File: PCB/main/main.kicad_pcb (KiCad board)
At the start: 2 copper layers, 82.3 x 36.1 mm, 38 parts, among them IC1 LT8316IFE#PBF, Q1 PBHV9050ZF, Q2 IXTA10P50P, Q3 SIHB24N80AE-GE3, T1 Transformer_1P_2S

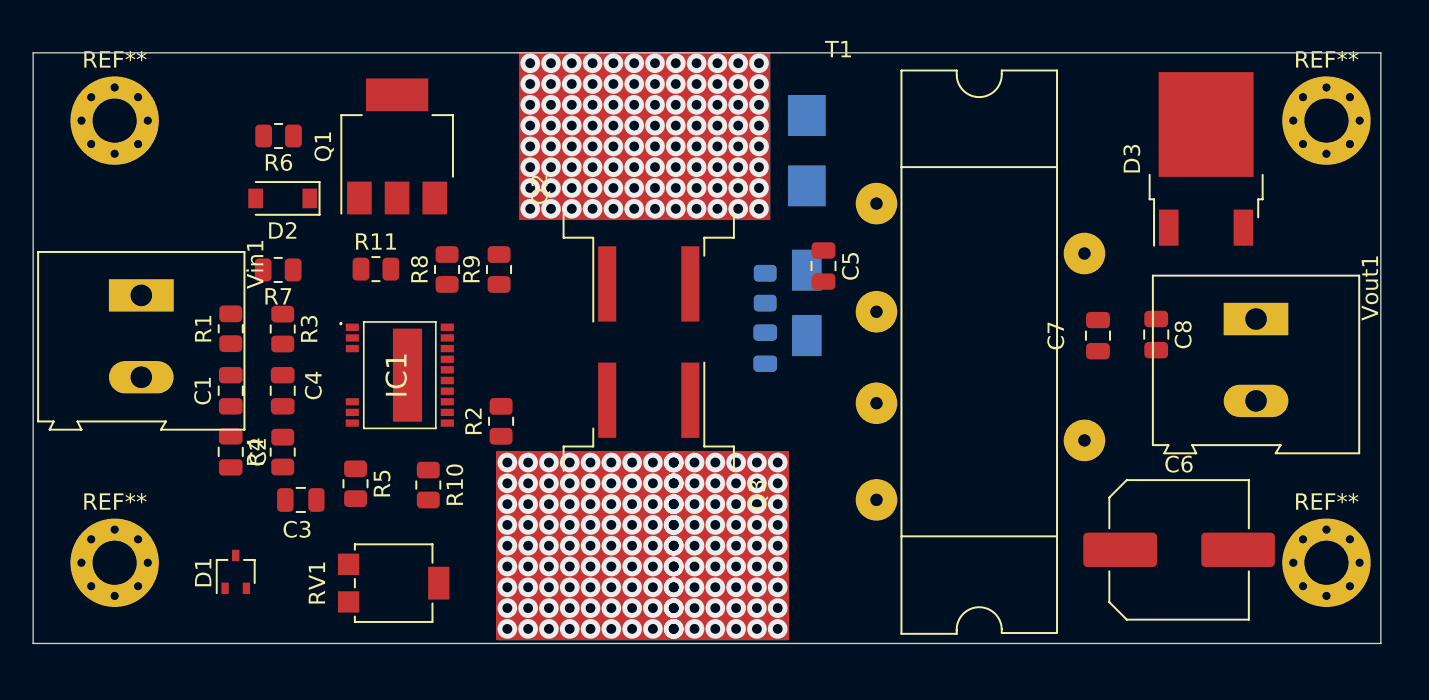
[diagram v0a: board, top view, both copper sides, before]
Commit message: pcb drawing update
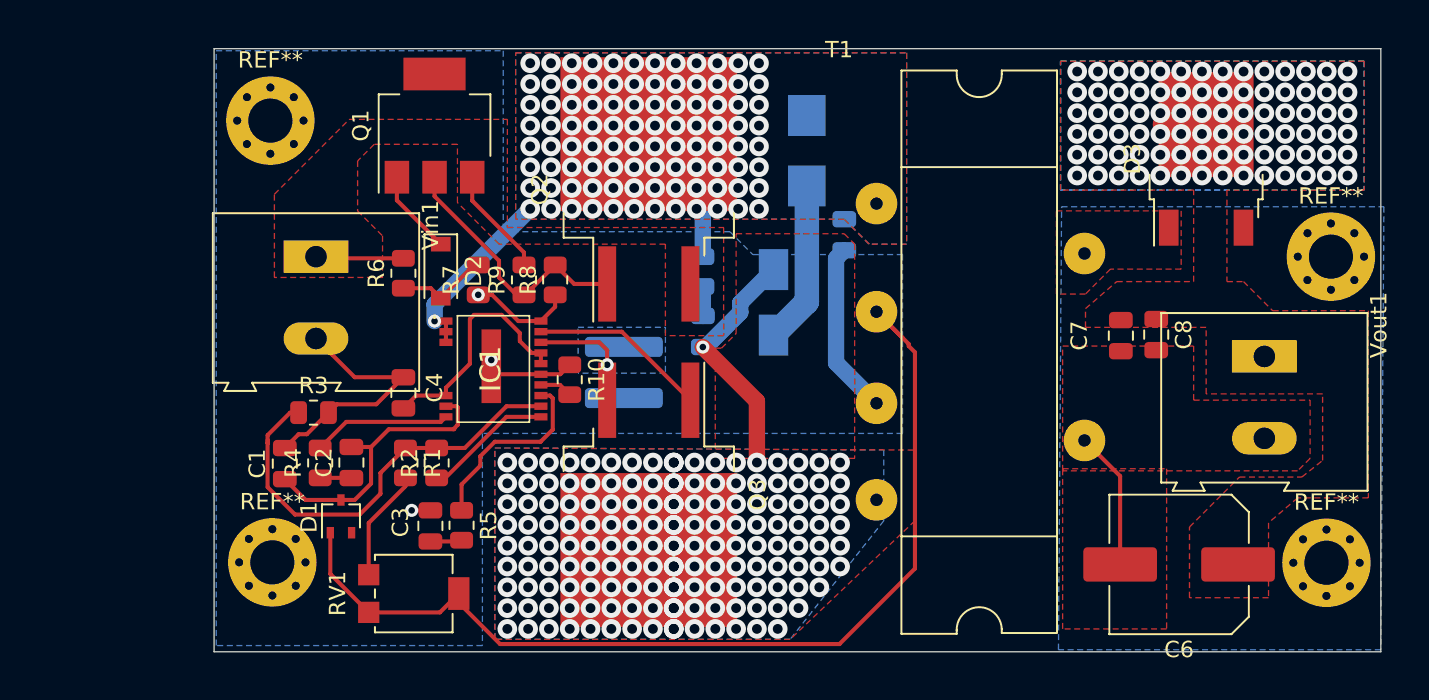
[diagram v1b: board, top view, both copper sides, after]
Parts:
- C5: moved to B.Cu
- R11: footprint Resistor_SMD:R_0805_2012Metric -> Resistor_SMD:R_1218_3246Metric_Pad1.22x4.75mm_HandSolder; moved to B.Cu
- moved R11 16.4 mm to (101.1, 42.4), turned to 90 degrees
- moved R1 13.5 mm to (87.8, 47.9), turned to 270 degrees
- moved R7 12.2 mm to (92.2, 36.7), turned to 90 degrees
- moved R6 11.3 mm to (87.6, 36.3), turned to 90 degrees
- moved Vin1 10.9 mm to (82.3, 35.3)
- moved R10 10.8 mm to (97.8, 42.8)
- moved D2 10.6 mm to (89.9, 36.2), turned to 270 degrees
- moved REF** 9.63 mm to (79.6, 54.0)
- moved REF** 9.51 mm to (79.5, 27.0)
- moved REF** 8.31 mm to (144.3, 35.3)
- moved C3 8.07 mm to (89.3, 51.8), turned to 270 degrees
- moved C2 7.39 mm to (84.5, 47.9), turned to 90 degrees
- moved C4 7.37 mm to (87.6, 43.6)
- moved D1 7.27 mm to (83.8, 51.2)
- moved R5 6.96 mm to (91.2, 51.7)
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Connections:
- D3 pad 1: Net-(C6-Pad1) -> Net-(D3-Pad1)
- D3 pad 2: Net-(D3-Pad2) -> Net-(C6-Pad1)
- D5 pad 1: Net-(D4-Pad1) -> Net-(C9-Pad2)
- D5 pad 2: Net-(C9-Pad2) -> Net-(D4-Pad1)
- T1 pad 3: Net-(D3-Pad2) -> Net-(D3-Pad1)
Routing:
- net V_FB: track 0.00 -> 62.1 mm
- net GND1: track 0.00 -> 42.0 mm, vias 0 -> 3
- net Net-(IC1-Pad12): track 0.00 -> 26.7 mm
- net Net-(C1-Pad1): track 0.00 -> 17.4 mm
- net Net-(Q1-Pad2): track 0.00 -> 16.0 mm
- net Net-(C9-Pad2): track 0.00 -> 15.0 mm, vias 80 -> 157
- net Net-(C4-Pad1): track 0.00 -> 14.5 mm
- net V_in: track 0.00 -> 14.4 mm, vias 71 -> 96
- net Net-(Q1-Pad3): track 0.00 -> 12.0 mm
- net Net-(IC1-Pad13): track 0.00 -> 11.6 mm
- net Net-(IC1-Pad19): track 0.00 -> 10.9 mm
- net Net-(D4-Pad1): track 0.00 -> 9.95 mm
- net Net-(IC1-Pad18): track 0.00 -> 9.85 mm, vias 0 -> 1
- net Net-(C6-Pad2): track 0.00 -> 8.47 mm
- net Net-(IC1-Pad10): track 0.00 -> 8.47 mm
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- added copper zone on B.Cu, net GND1
- added copper zone on B.Cu, net Net-(C6-Pad1)
- added copper zone on F.Cu, net Net-(C6-Pad1)
- added copper zone on B.Cu, net Net-(C6-Pad2)
- added copper zone on F.Cu, net Net-(C6-Pad2)
- added copper zone on B.Cu, net Net-(C9-Pad2)
- added copper zone on F.Cu, net Net-(C9-Pad2)
- added copper zone on F.Cu, net Net-(D3-Pad1)
- added copper zone on B.Cu, net Net-(D3-Pad2)
- added copper zone on B.Cu, net Net-(IC1-Pad18)
- added copper zone on F.Cu, net Net-(Q1-Pad3)
- added copper zone on B.Cu, net V_in
- added copper zone on F.Cu, net V_in
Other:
- board size 82.3 x 36.1 mm -> 71.2 x 36.8 mm
- net class T_1.5 added: clearance 0.2, trace_width 1.5, via_dia 1, via_drill 0.6
